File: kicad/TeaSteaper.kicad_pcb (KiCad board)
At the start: 2 copper layers, 100 x 60 mm, 16 parts, among them J1 Serial, J2 JTAG, J3 Power +5v, J4 Display, J5 Stepper, SW2 Rotary_Encoder_Switch, U1 ESP32-WROOM-32D, U2 ULN2803A, U3 AH3572-SA-7, U5 AZ1117-3.3

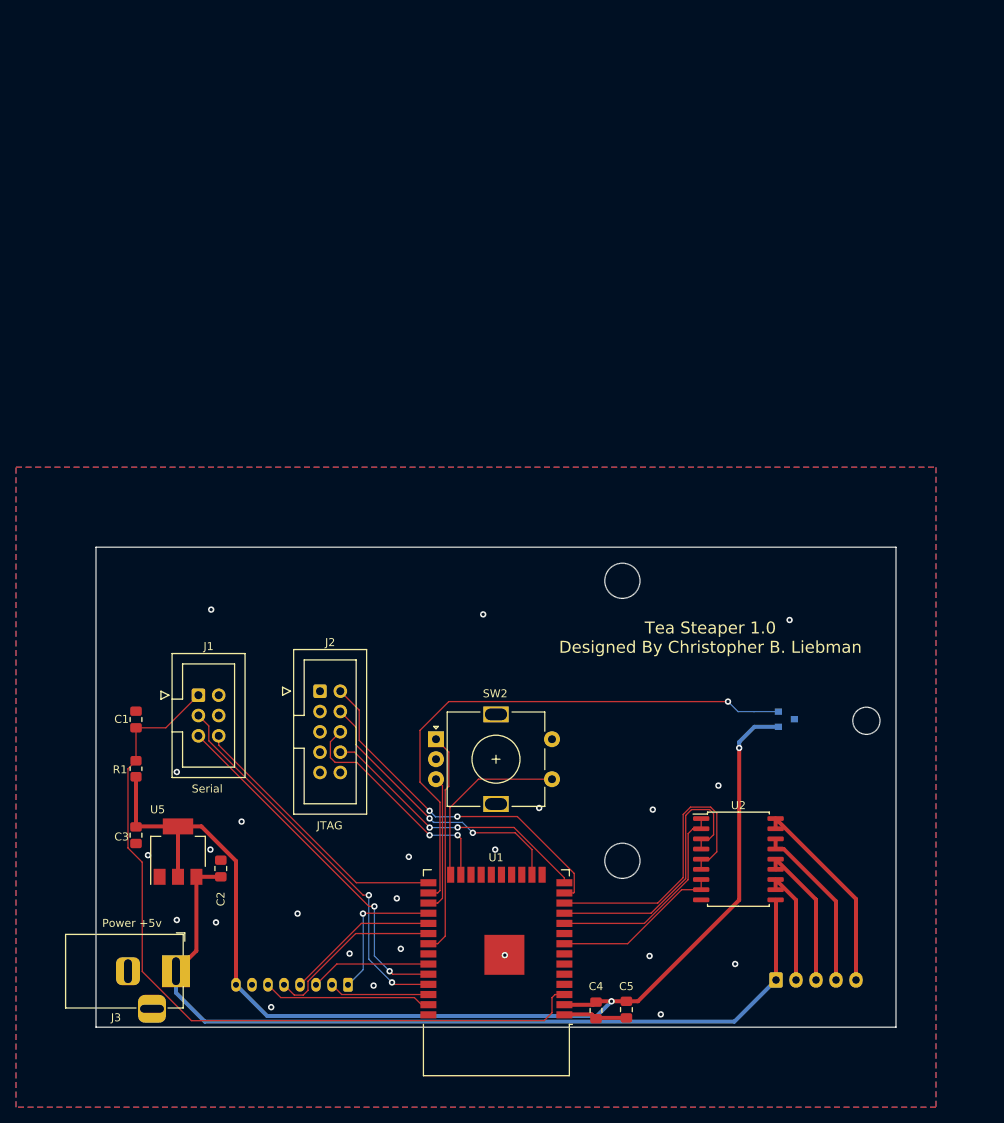
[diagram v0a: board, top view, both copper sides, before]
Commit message: board v1.1
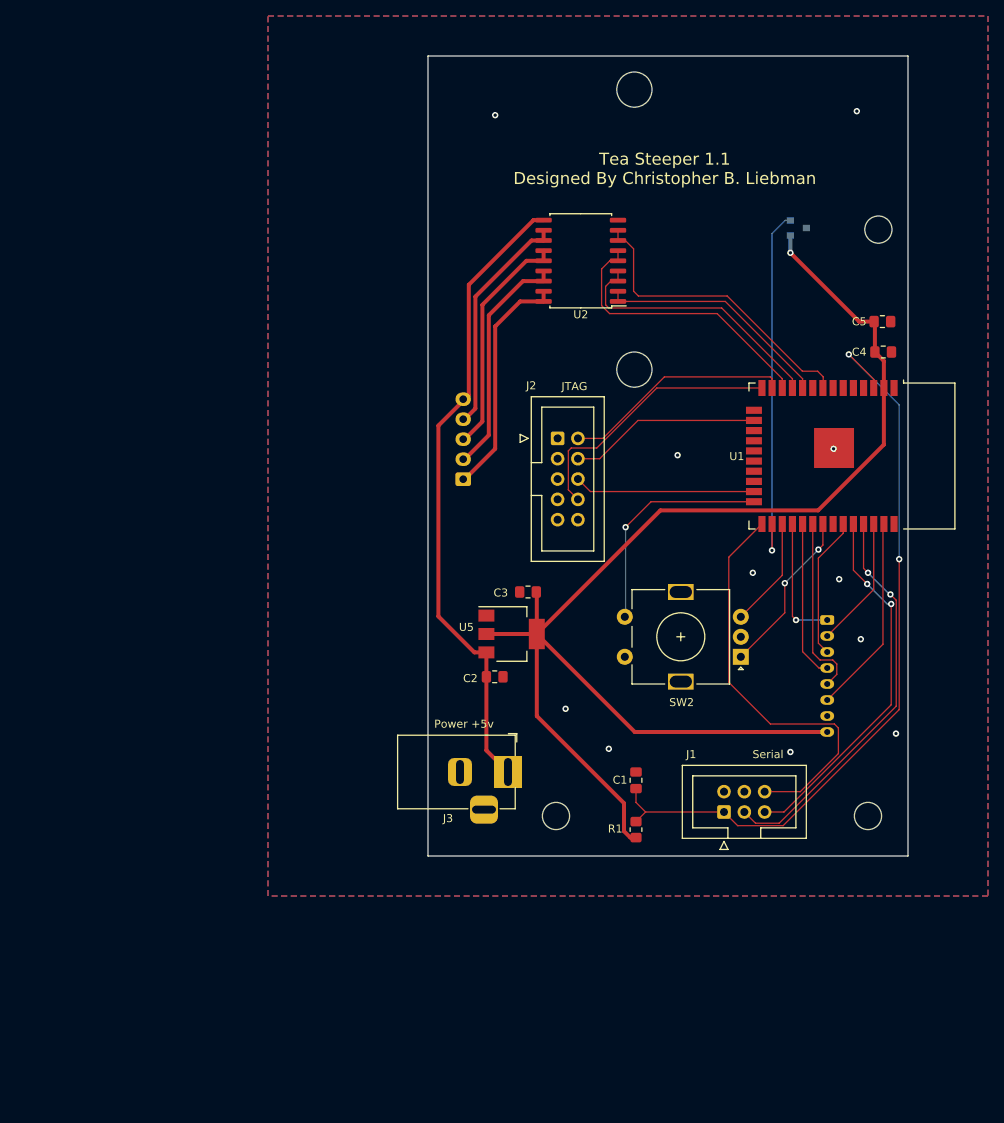
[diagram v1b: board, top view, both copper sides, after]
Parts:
- moved C5 91.8 mm to (191.0, 66.6), turned to 0 degrees
- moved C4 89.8 mm to (191.1, 70.4), turned to 0 degrees
- moved U2 77.4 mm to (153.3, 59.0), turned to 180 degrees
- moved J4 75.3 mm to (184.1, 103.9), turned to 270 degrees
- moved U1 74.2 mm to (184.2, 83.4), turned to 270 degrees
- moved J5 73.8 mm to (138.6, 86.3), turned to 90 degrees
- moved J1 67.3 mm to (171.2, 127.9), turned to 90 degrees
- moved C1 63.0 mm to (160.2, 123.9)
- moved R1 63.0 mm to (160.2, 130.1)
- moved U3 61.4 mm to (180.5, 54.9)
- moved C3 57.7 mm to (146.7, 100.4), turned to 180 degrees
- moved U5 49.8 mm to (144.7, 105.6), turned to 0 degrees
- moved J3 48.4 mm to (144.2, 122.9)
- moved J2 43.4 mm to (150.4, 81.2)
- moved C2 41.8 mm to (142.5, 111.0), turned to 0 degrees
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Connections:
- J5 pad 1: +5V -> /P_M1A
- J5 pad 2: /P_M1D -> /P_M1B
- J5 pad 4: /P_M1B -> /P_M1D
- J5 pad 5: /P_M1A -> +5V
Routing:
- net +5V: track 107.3 -> 79.7 mm
- net +3V3: track 144.4 -> 169.2 mm, vias 2 -> 1
- net /ULIM: track 69.4 -> 45.9 mm
- net /IO0: track 34.5 -> 52.0 mm
- net /M1D: track 21.2 -> 38.5 mm
- net /TMS: track 44.5 -> 28.7 mm, vias 2 -> 0
- net /P_M1D: track 14.9 -> 28.7 mm
- net /TCK: track 35.5 -> 24.0 mm, vias 2 -> 0
- net /P_M1C: track 18.5 -> 29.1 mm
- net GND: track 8.04 -> 0.00 mm, vias 24 -> 11
- net /P_M1B: track 21.4 -> 29.3 mm
- net /ROTA: track 28.0 -> 20.9 mm, vias 0 -> 2
- net /TDO: track 28.8 -> 22.7 mm, vias 2 -> 0
- net /ROTSW: track 22.7 -> 28.6 mm, vias 0 -> 1
- net /RST: track 12.6 -> 16.4 mm
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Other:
- board size 100 x 60 mm -> 60 x 100 mm
- board text added: "Tea Steeper 1.1 Designed By Christopher B. Liebman"
- board text removed: "Tea Steaper 1.0 Designed By Christopher B. Liebman"
